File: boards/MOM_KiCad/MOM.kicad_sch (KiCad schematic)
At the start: 27 parts, among them J1 JST-PH, J2 USB_C_Receptacle_USB2.0, Q1 DMG3415U, SW1 SW_Push, SW2 SW_Push, U1 AP2112K-3.3, U2 MCP73831-2-OT, U3 LC709204F, U4 ESP32-S3-MINI-1

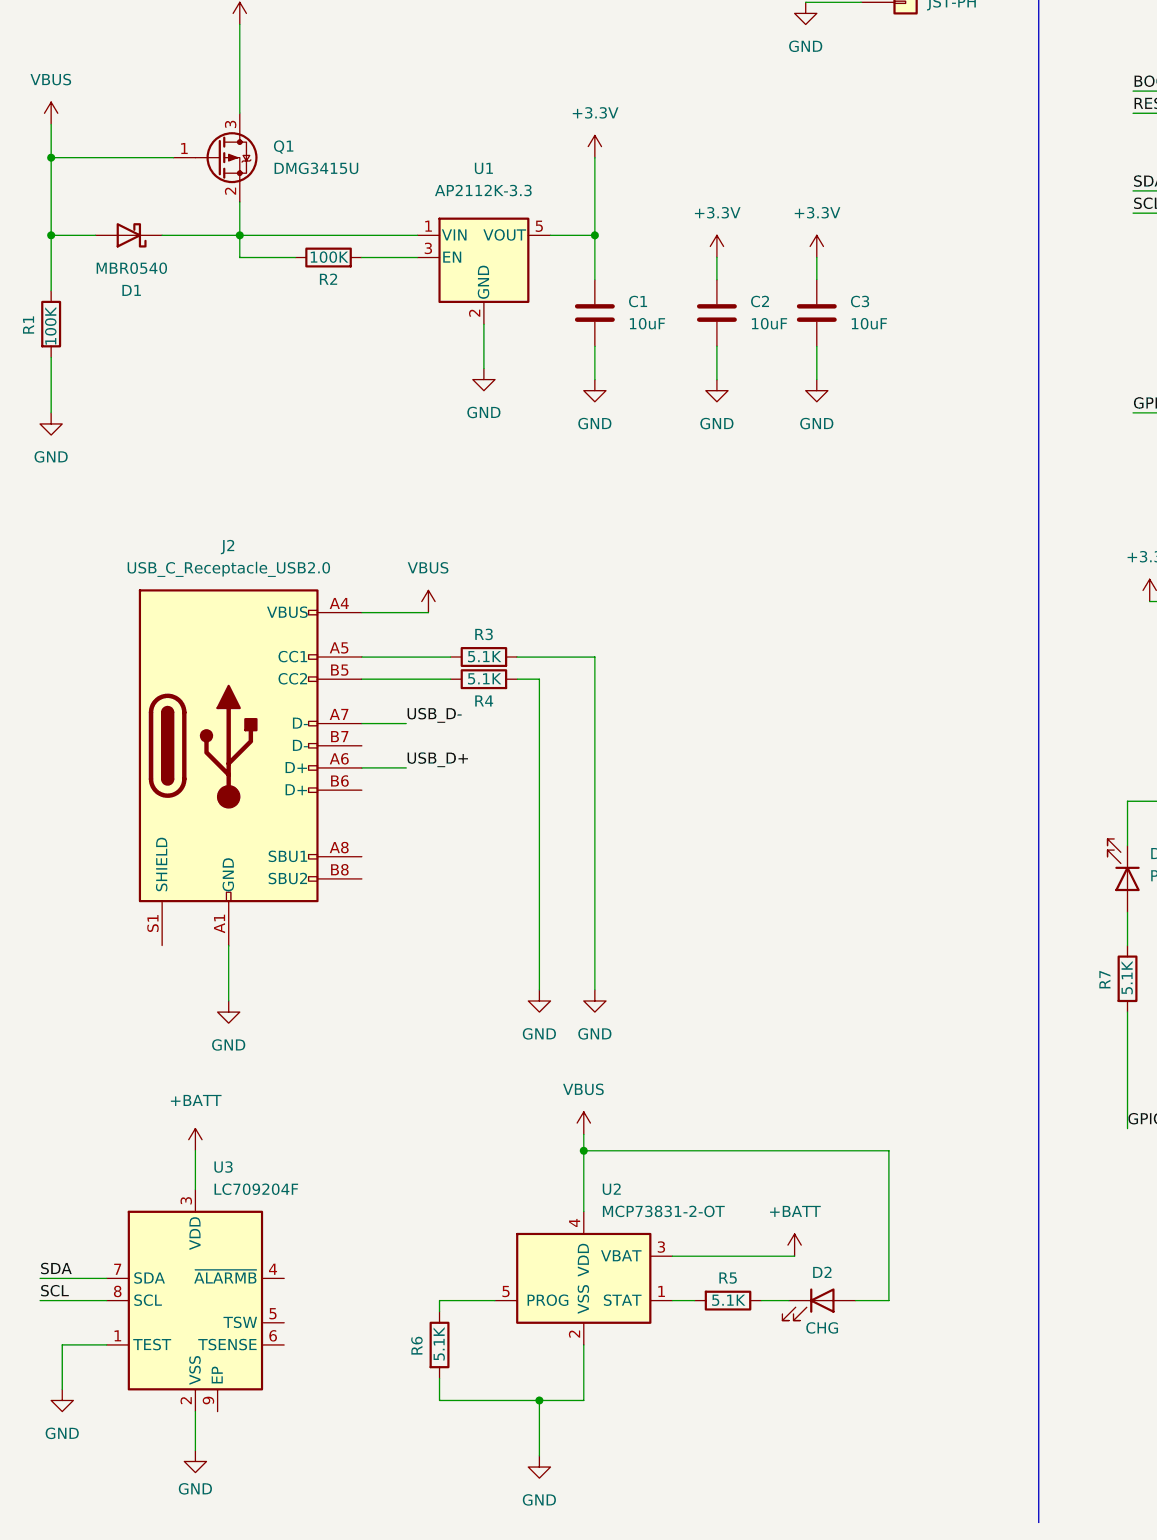
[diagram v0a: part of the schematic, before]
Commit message: New schematic revision and repo cleanup
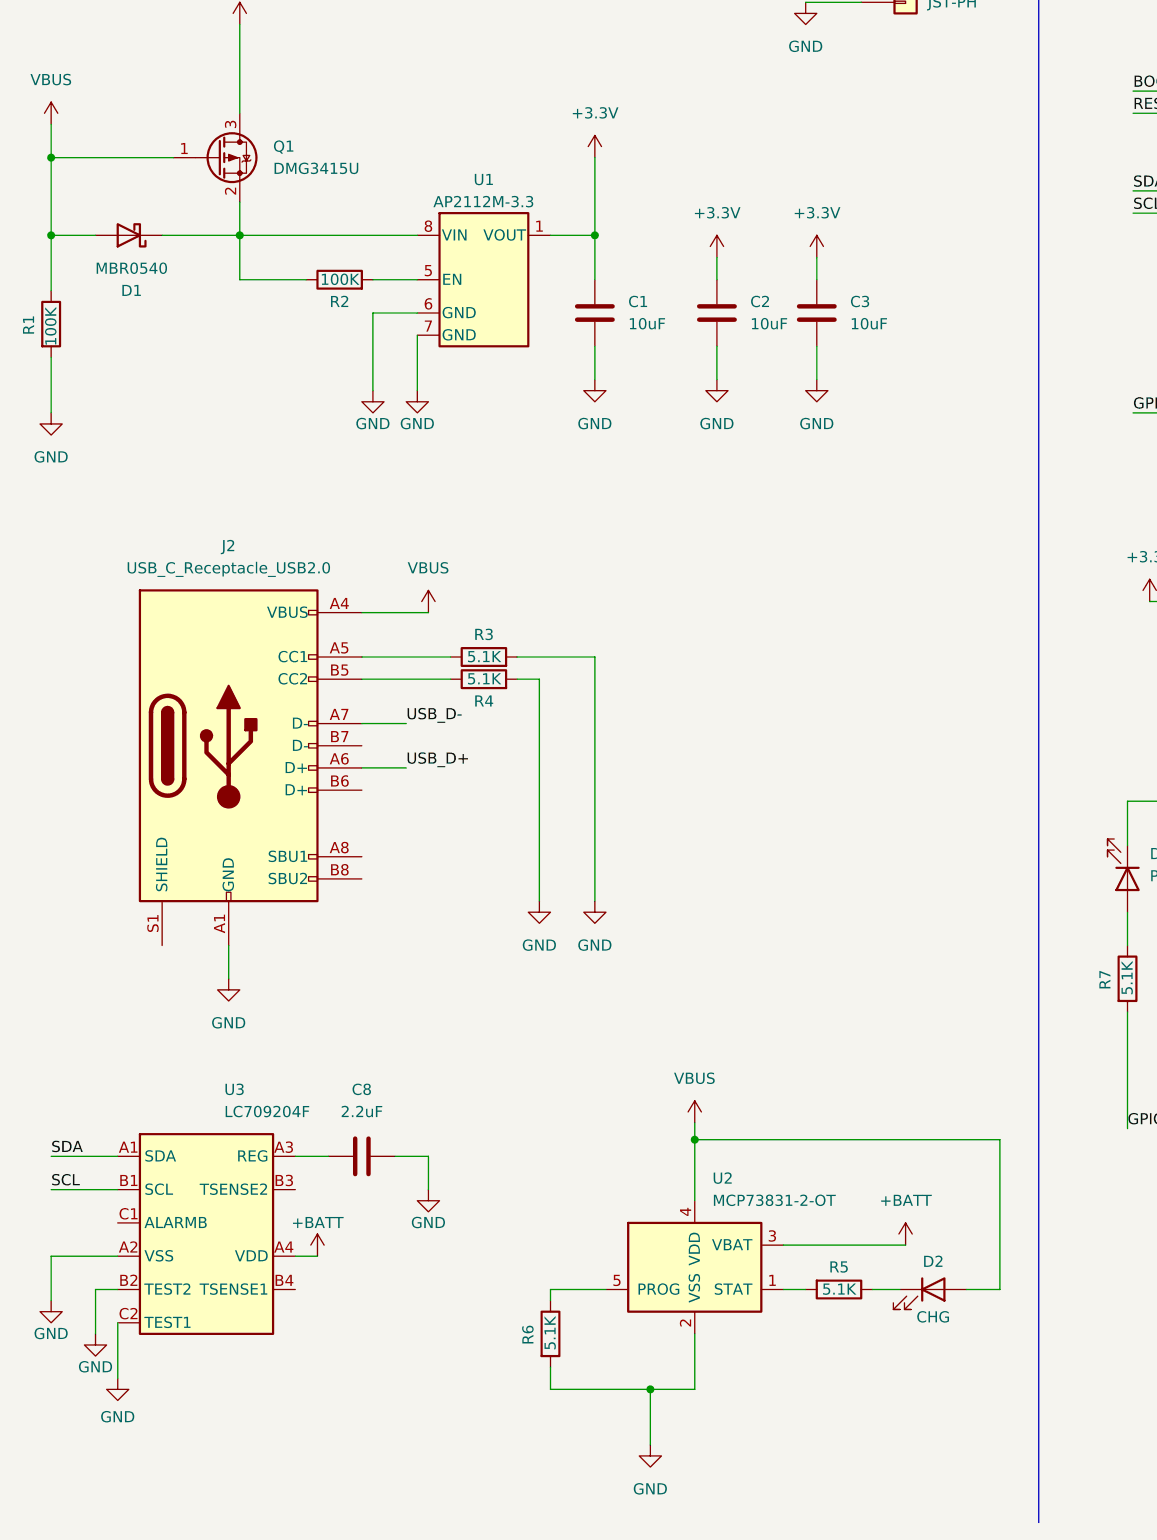
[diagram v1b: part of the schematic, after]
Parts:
- added C8: 2.2uF, symbol Device:C
- U1: value AP2112K-3.3 -> AP2112M-3.3; footprint Package_TO_SOT_SMD:SOT-23-5 -> Package_SO:Diodes_SO-8EP
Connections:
- net +3.3V: now also U1.1 (VOUT); no longer U1.5 (VOUT)
- net +BATT: now also U3.A4 (VDD); no longer U3.3 (VDD)
- net GND: now also U1.6 (GND), U1.7 (GND), U3.A2 (VSS), U3.B2 (TEST2), U3.C2 (TEST1), C8.2; no longer U1.2 (GND), U3.1 (TEST), U3.2 (VSS)
- net SCL: now also U3.B1 (SCL); no longer U3.8 (SCL)
- net SDA: now also U3.A1 (SDA); no longer U3.7 (SDA)
- net at D1.1 (K), Q1.2 (S), R2.1: now also U1.8 (VIN); no longer U1.1 (VIN)
- net at U1.3 (NC): no longer R2.2
- new net: R2.2, U1.5 (EN)
- new net: C8.1, U3.A3 (REG)
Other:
- moved on the sheet: D2, R2, R5, R6, U2
